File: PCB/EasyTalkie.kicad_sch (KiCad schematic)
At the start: 8 parts, among them J1 Battery, SW1 SW_Push, U1 XIAO-ESP32-S3-DIP, U2 INMP441, U3 MAX98357A

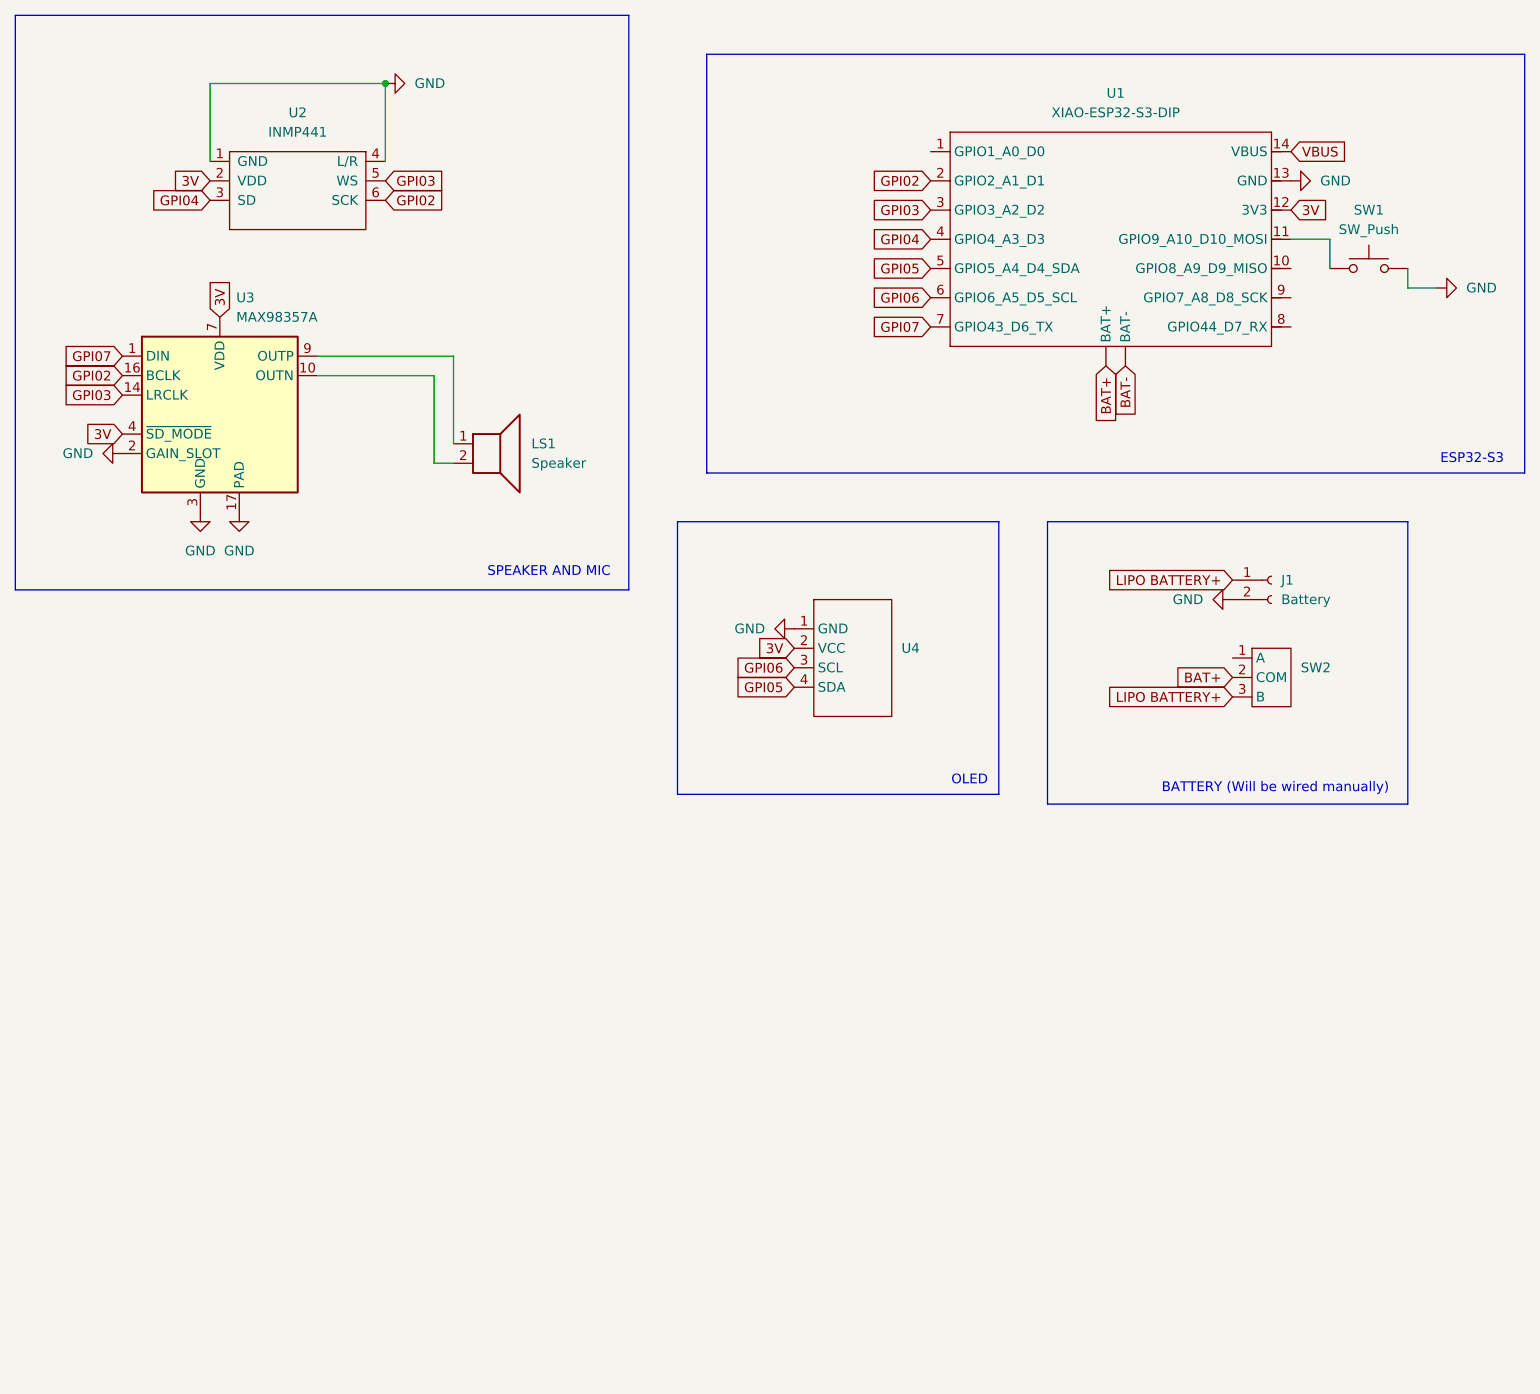
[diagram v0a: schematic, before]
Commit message: pcb
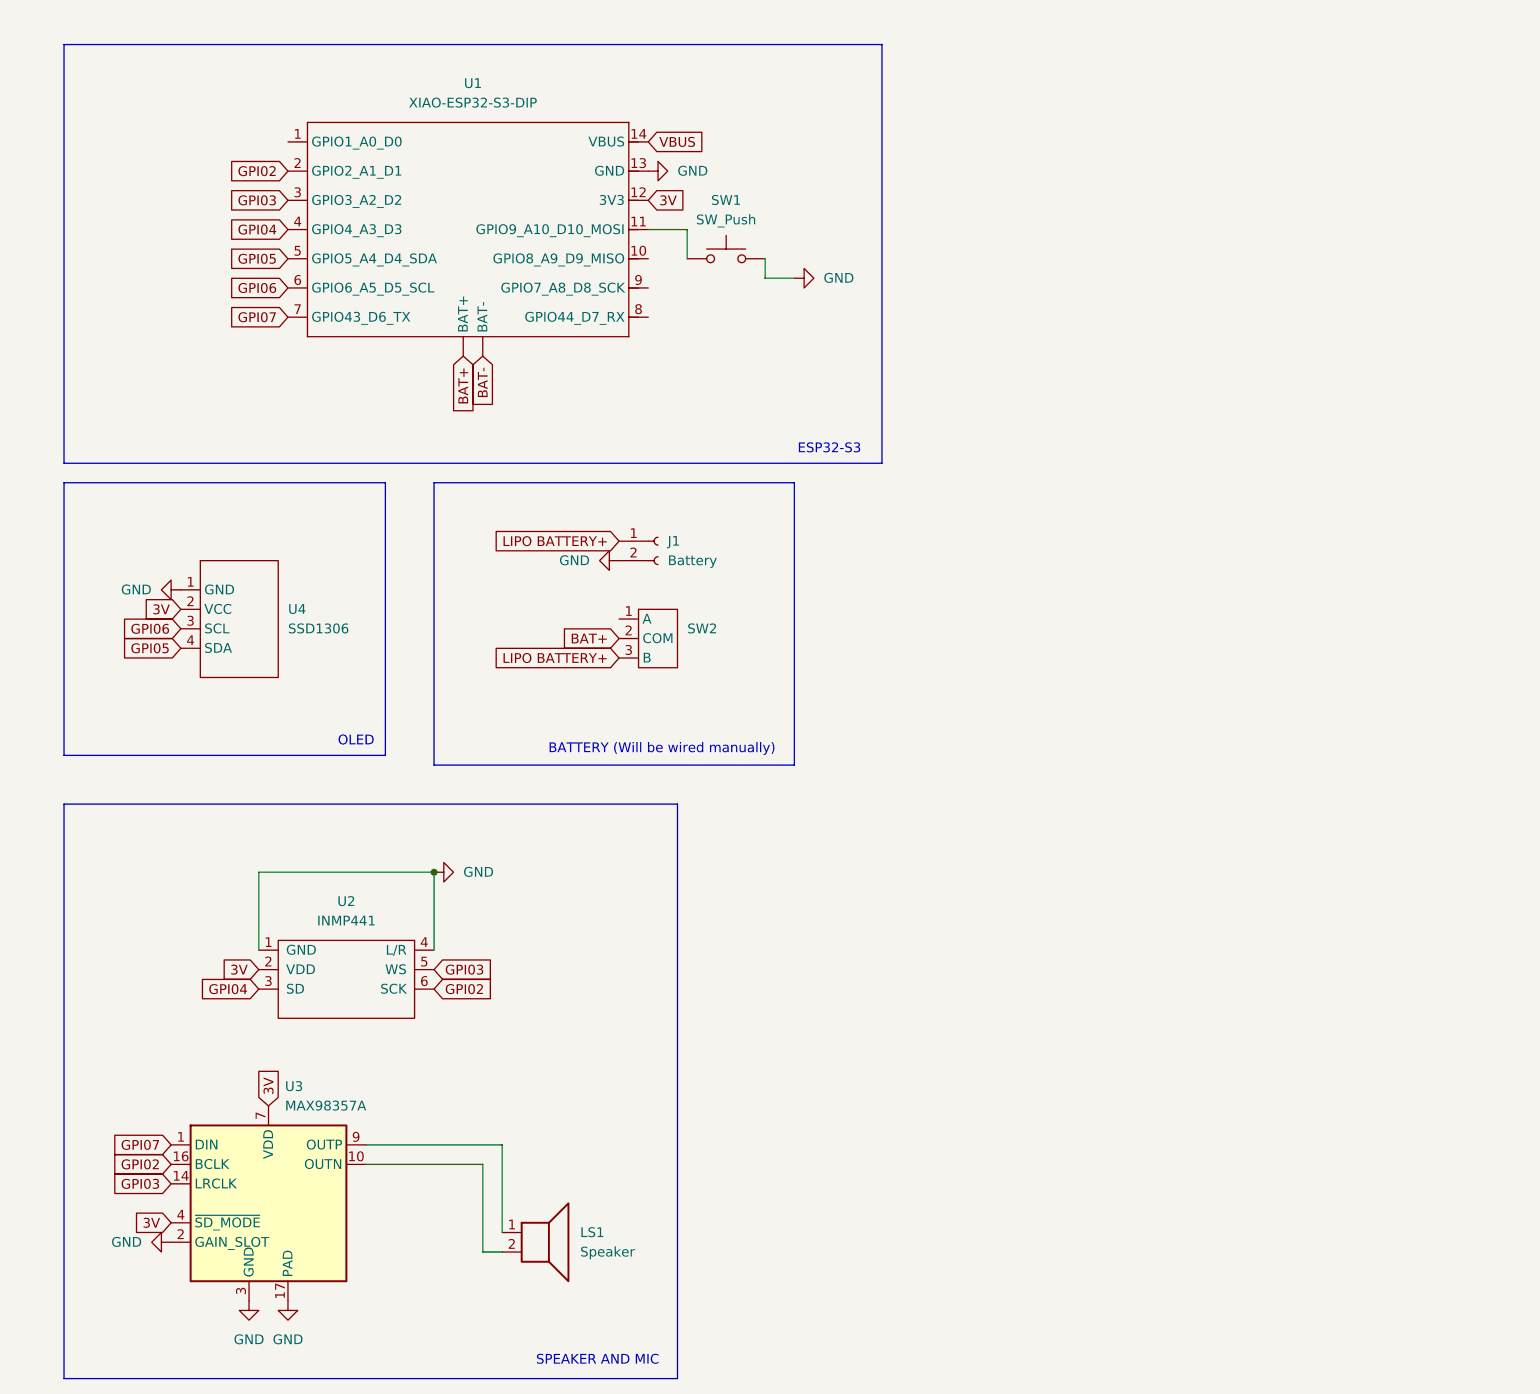
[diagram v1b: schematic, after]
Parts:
- U4: value ~ -> SSD1306
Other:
- moved on the sheet: J1, LS1, SW1, SW2, U1, U2, U3, U4

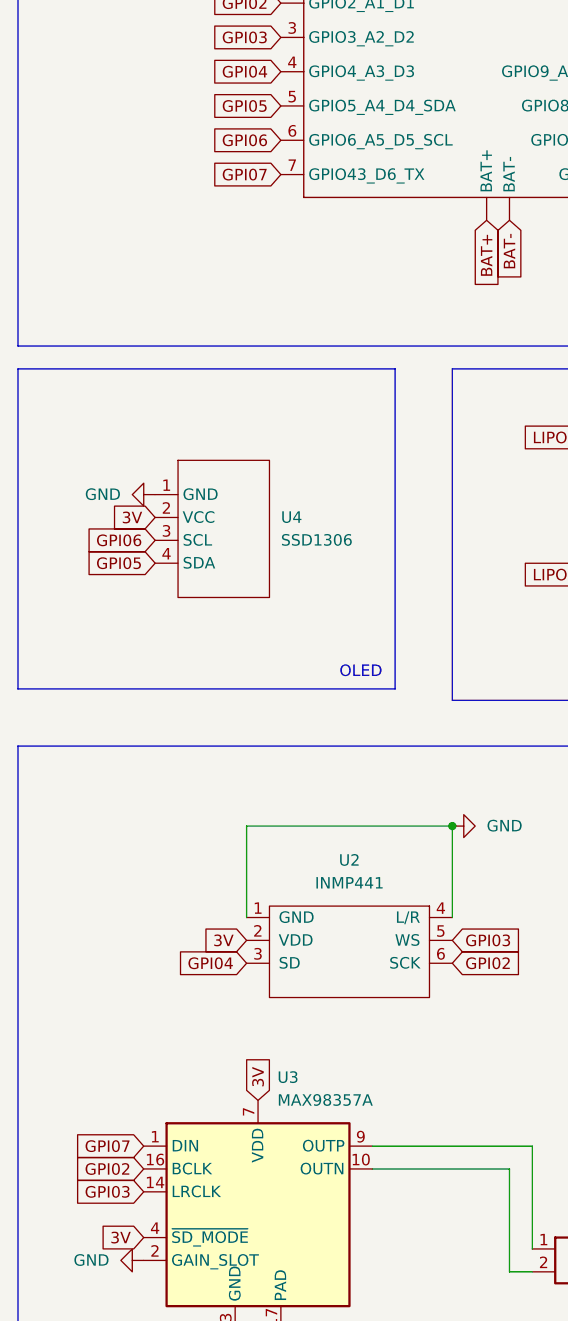
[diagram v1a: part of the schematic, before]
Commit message: firmware
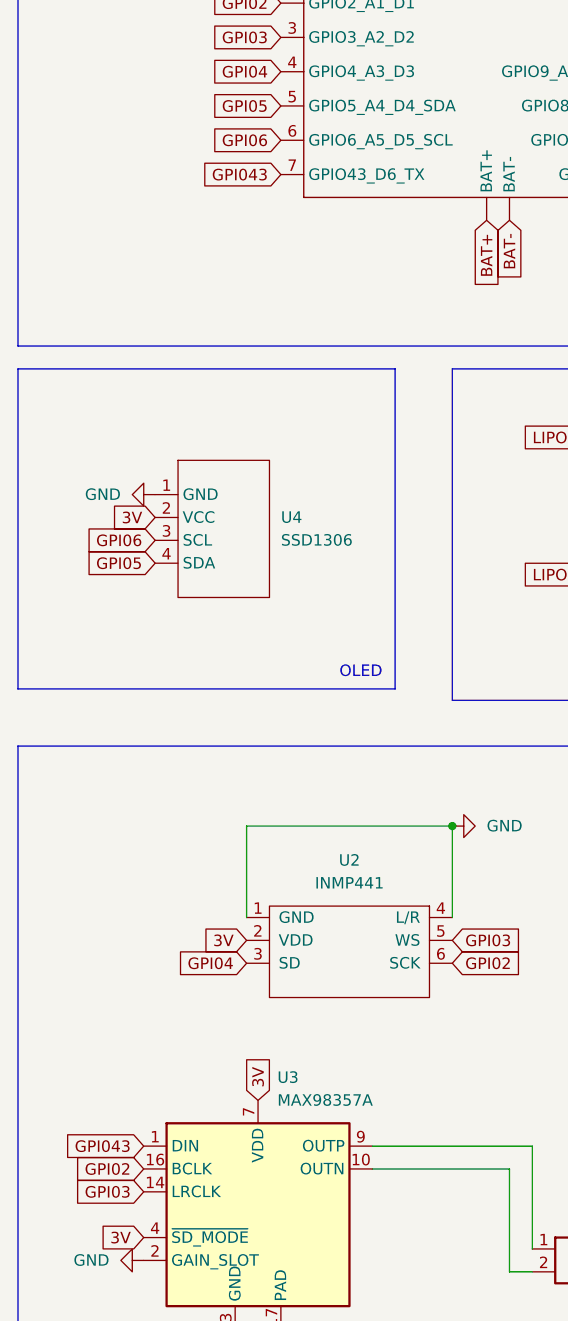
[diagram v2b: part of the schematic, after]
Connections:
- net GPI07 renamed GPI043
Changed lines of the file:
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@@
 		)
 	)
-	(global_label "GPI07"
+	(global_label "GPI043"
 		(shape input)
 		(at 50.8 54.61 180)
@@
 		)
 		(property "Intersheetrefs" "${INTERSHEET_REFS}"
-			(at 42.251 54.61 0)
+			(at 41.0415 54.61 0)
 			(effects
 				(font
@@
 		)
 	)
-	(global_label "GPI07"
+	(global_label "GPI043"
 		(shape input)
 		(at 35.56 162.56 180)
@@
 		)
 		(property "Intersheetrefs" "${INTERSHEET_REFS}"
-			(at 27.011 162.56 0)
+			(at 25.8015 162.56 0)
 			(effects
 				(font

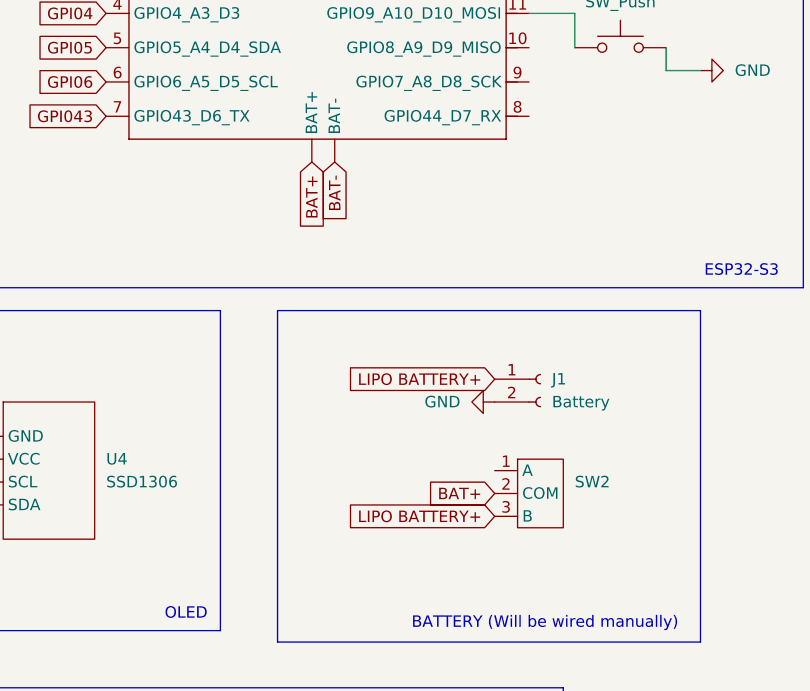
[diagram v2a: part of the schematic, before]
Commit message: fix
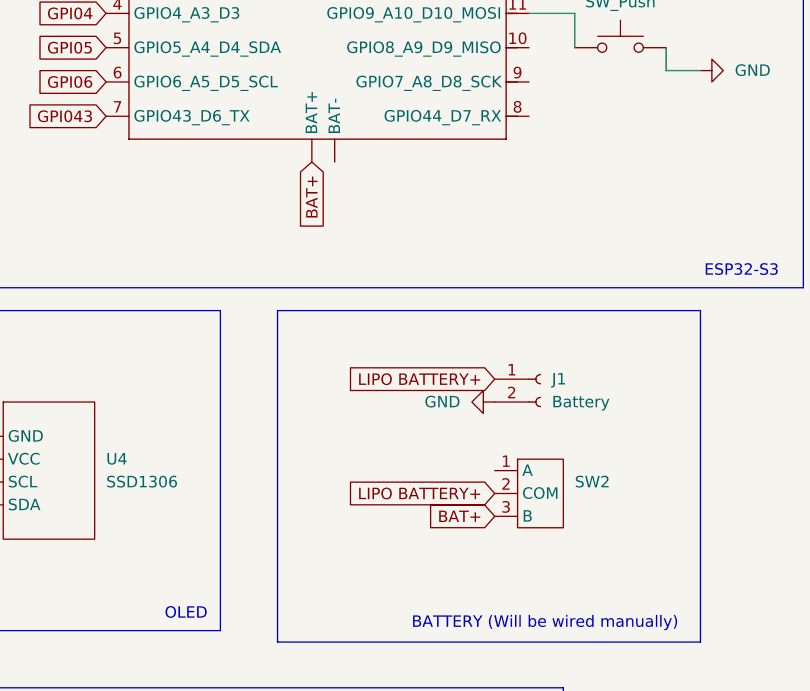
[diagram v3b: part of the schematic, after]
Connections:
- net BAT- is gone; now on net BAT+: U1. (BAT-)
- net BAT+: now also SW2.3 (B); no longer SW2.2 (COM)
- net LIPO BATTERY+: now also SW2.2 (COM); no longer SW2.3 (B)
